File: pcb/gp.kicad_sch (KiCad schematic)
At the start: 31 parts, among them J1 USB-C, SW1 TS-1088R-02526, SW2 TS-1088R-02526, U1 XC6206P332MR, U2 STM32F103CBT6, U3 W25Q32JVSS, Y1 16Mhz

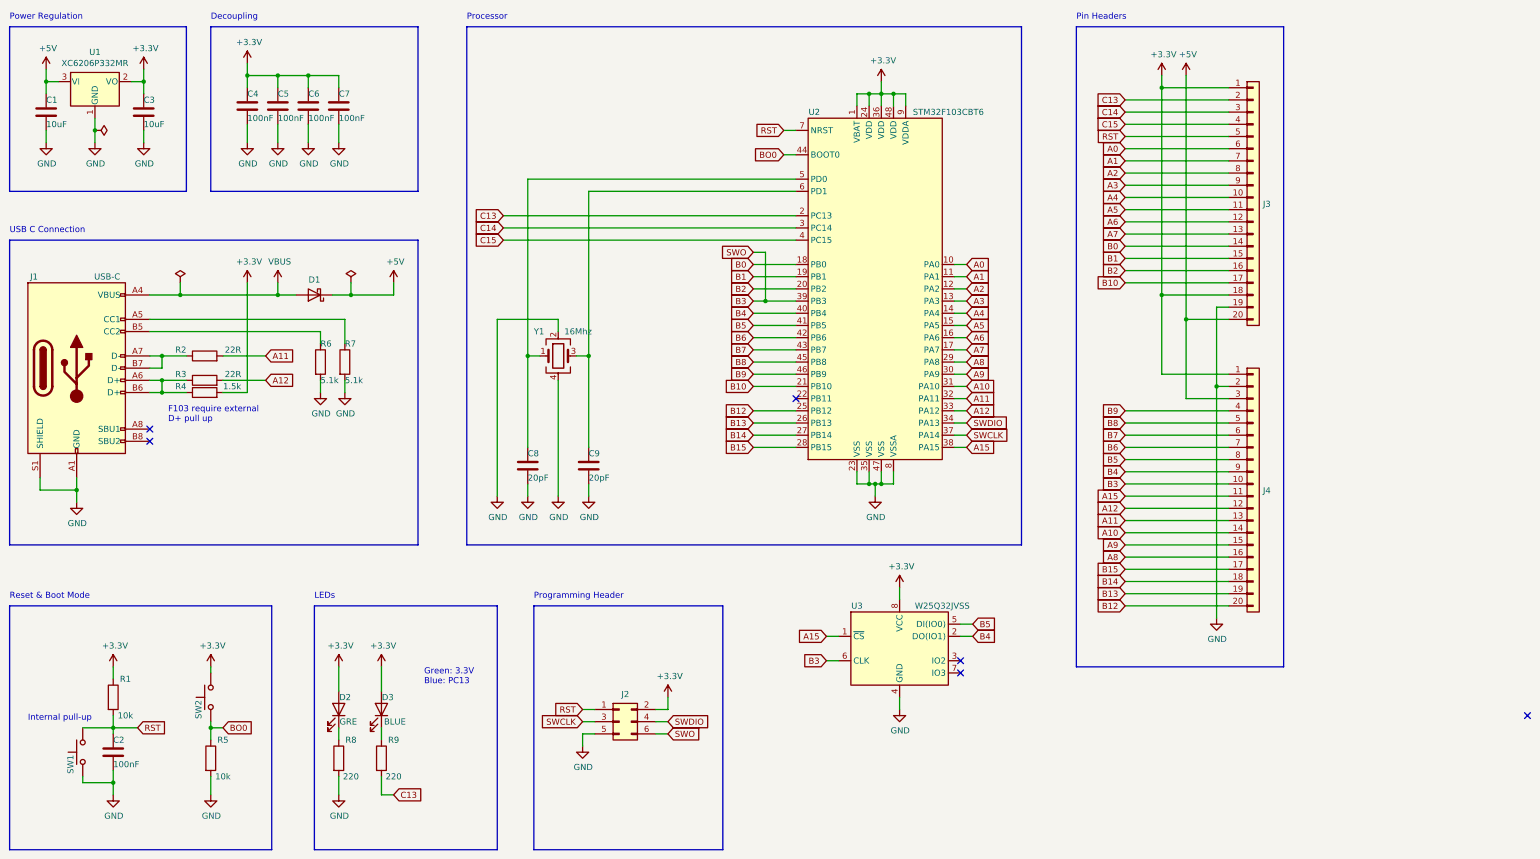
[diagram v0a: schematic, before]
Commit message: Hmmm
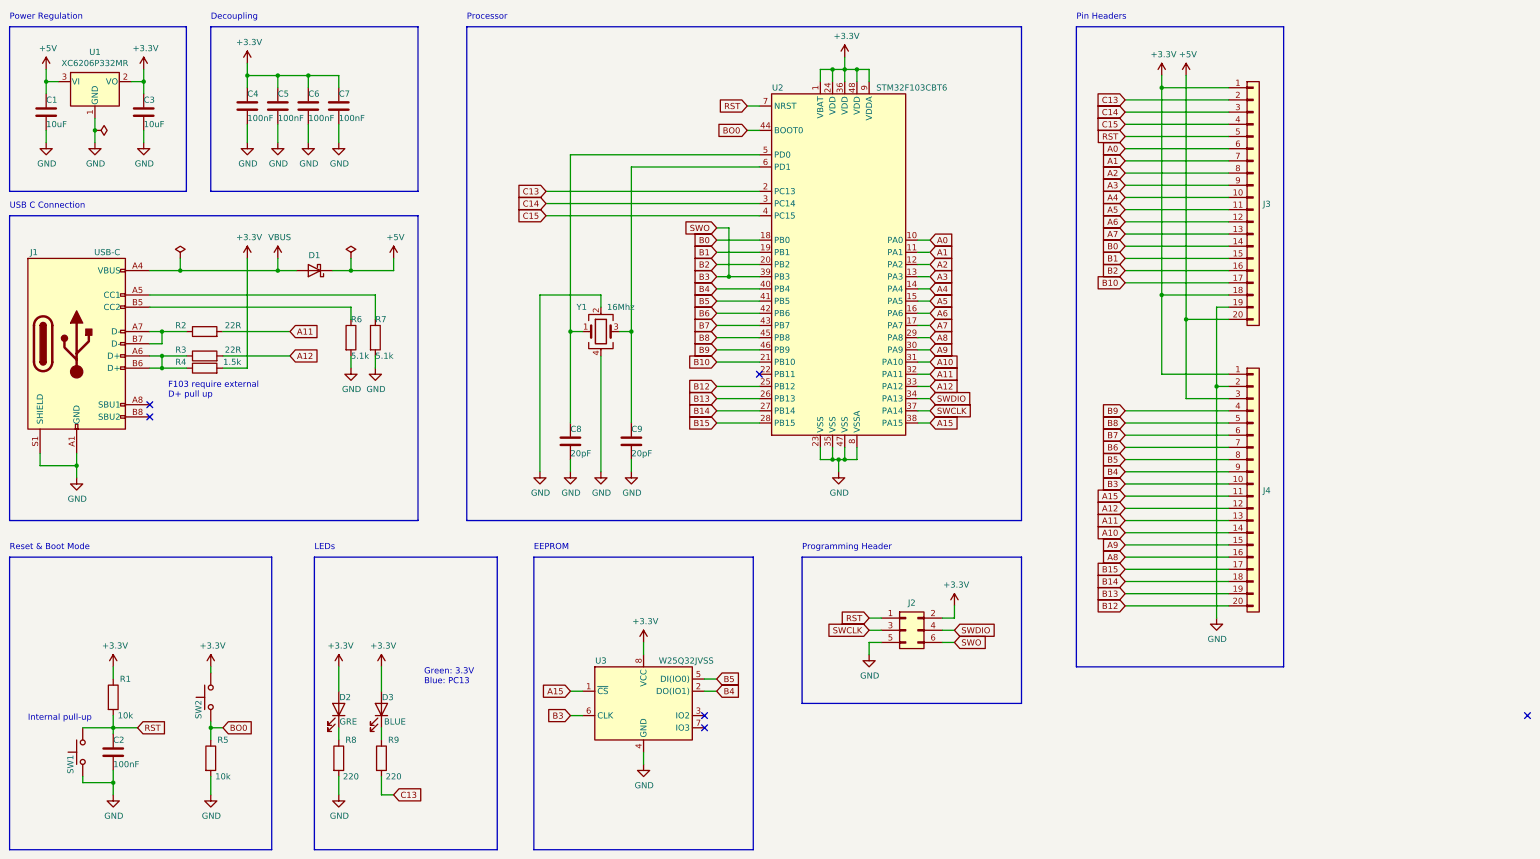
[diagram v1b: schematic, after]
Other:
- note added: "EEPROM"
- moved on the sheet: C8, C9, D1, J1, J2, R2, R3, R4, R6, R7, U2, U3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

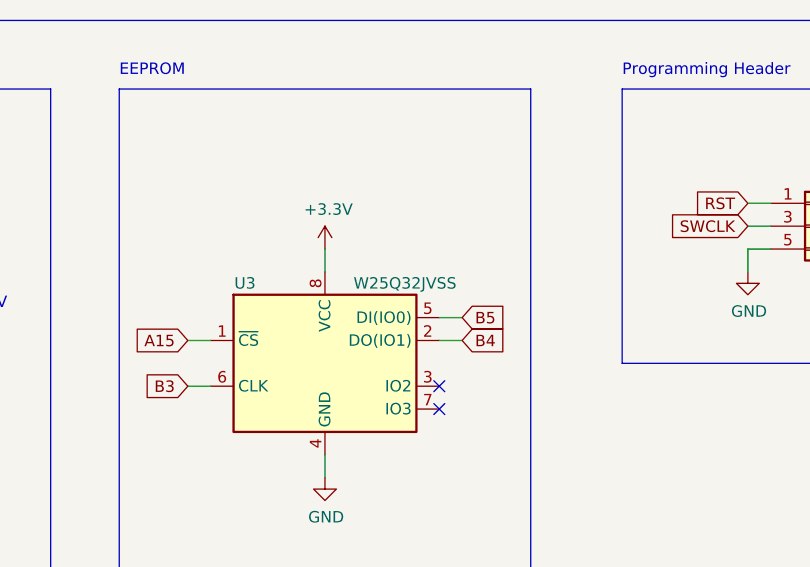
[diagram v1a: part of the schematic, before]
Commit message: Hmmmm
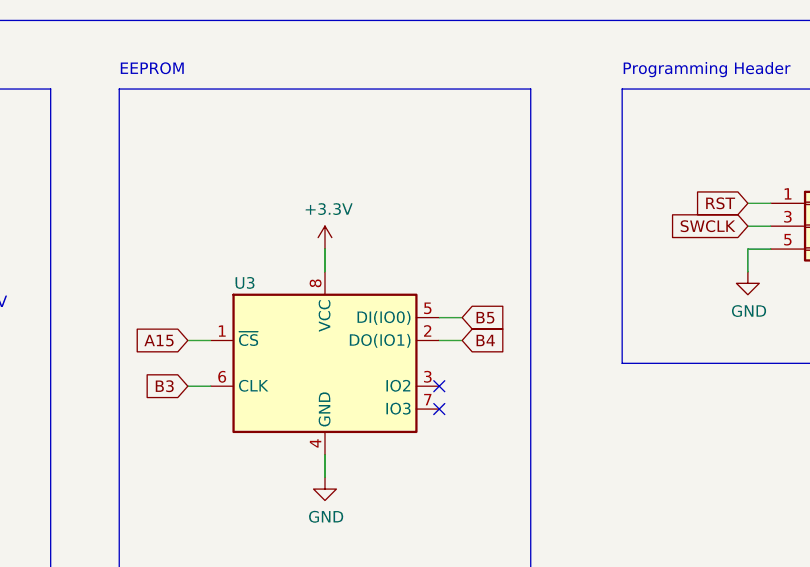
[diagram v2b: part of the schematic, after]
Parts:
- U3: value W25Q32JVSS -> (none); footprint Package_SO:SOIC-8_5.23x5.23mm_P1.27mm -> (none)
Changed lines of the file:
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@@
     (in_bom yes) (on_board yes)
     (property "Reference" "U3" (id 0) (at 137.16 149.86 0))
-    (property "Value" "W25Q32JVSS" (id 1) (at 154.94 149.86 0))
-    (property "Footprint" "Package_SO:SOIC-8_5.23x5.23mm_P1.27mm" (id 2) (at 146.05 158.75 0)
+    (property "Value" "" (id 1) (at 154.94 149.86 0))
+    (property "Footprint" "" (id 2) (at 146.05 158.75 0)
       (effects (font (size 1.27 1.27)) hide)
     )

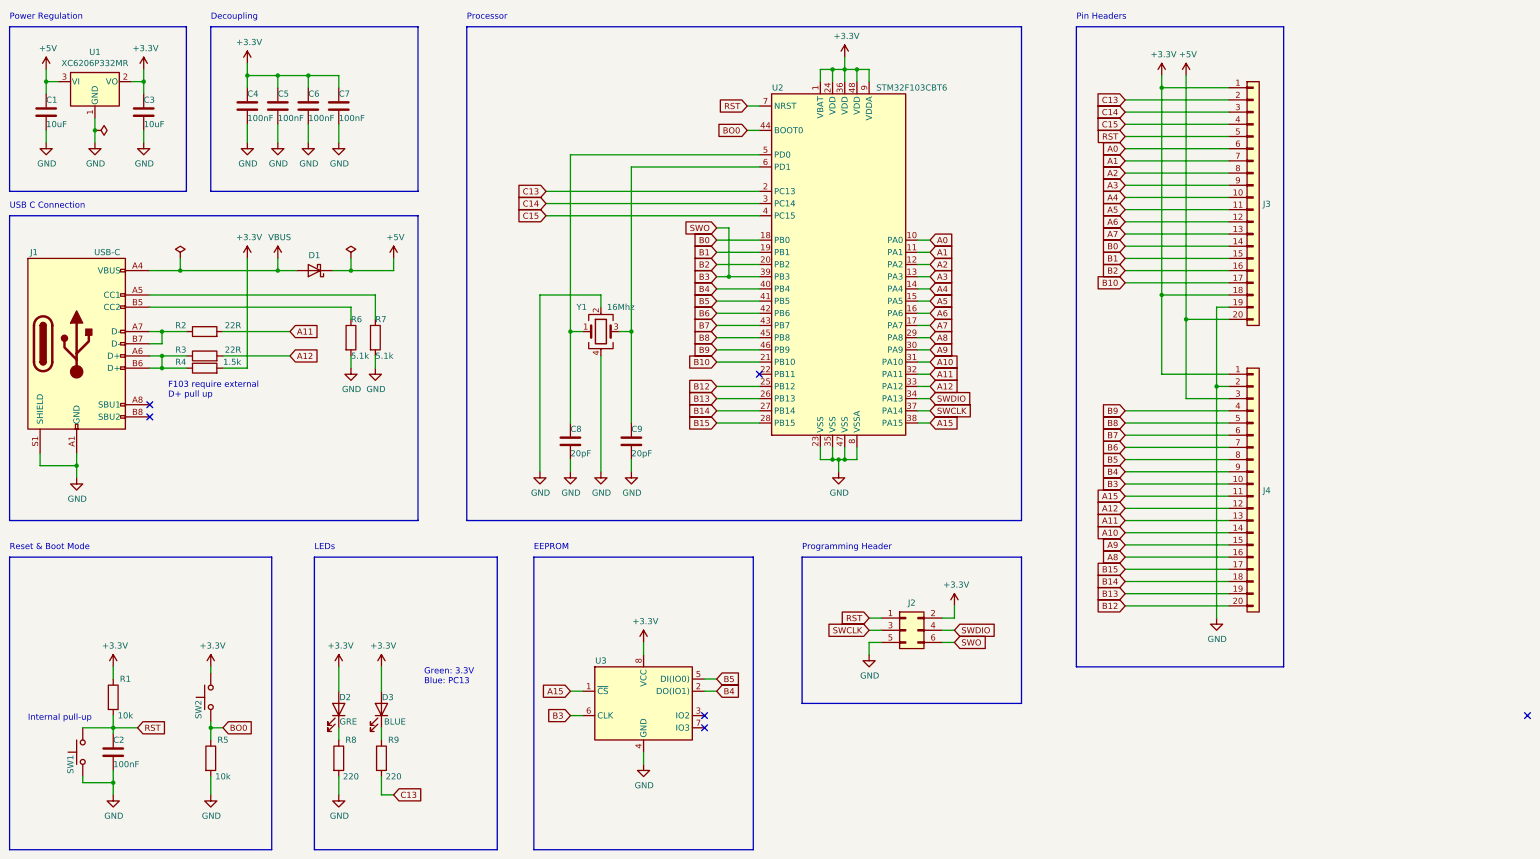
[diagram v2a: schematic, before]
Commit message: Tweaking
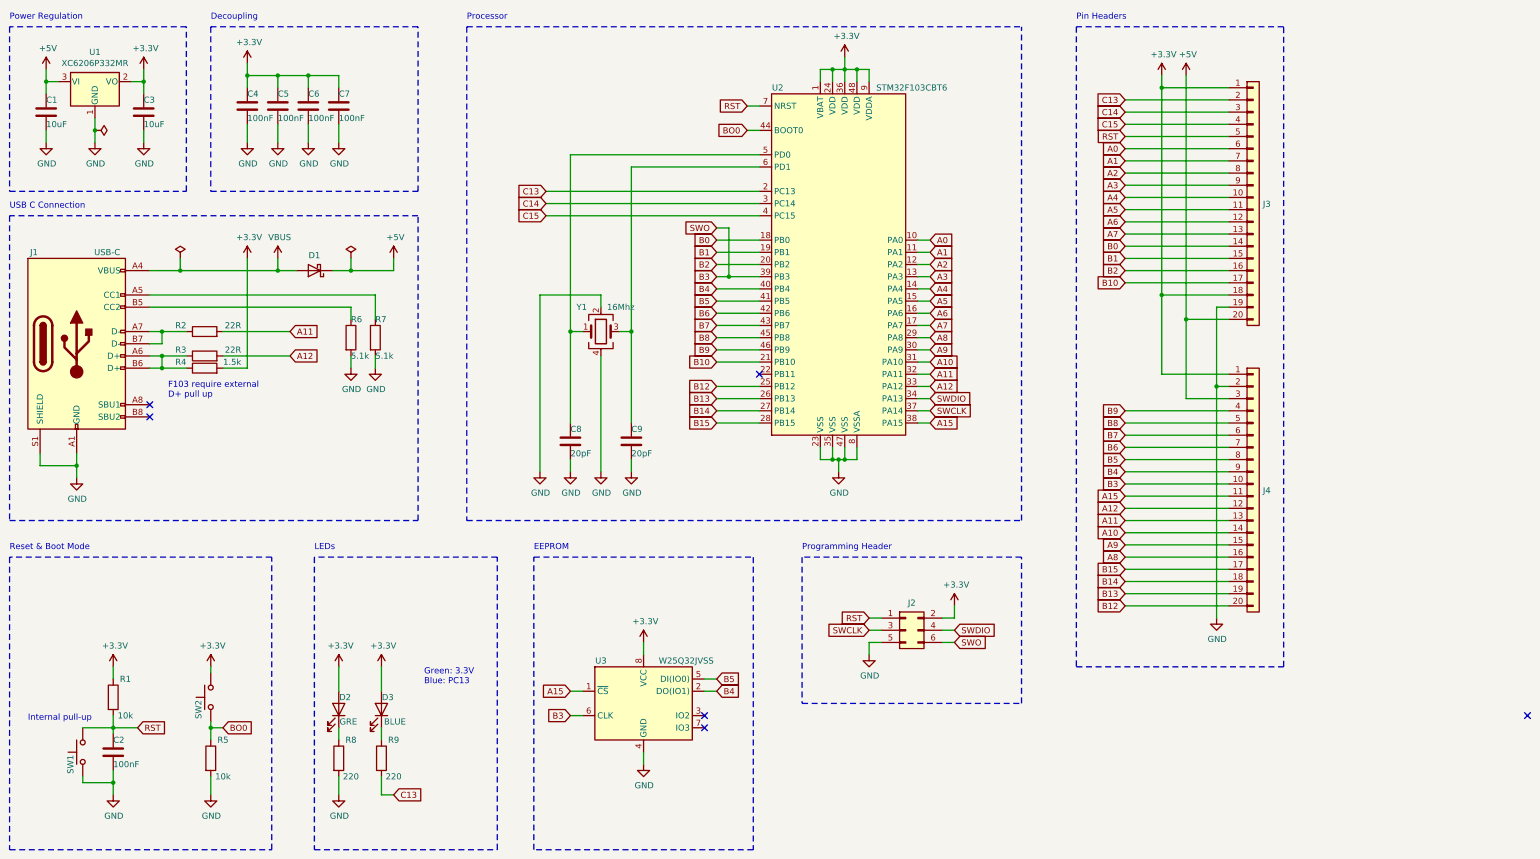
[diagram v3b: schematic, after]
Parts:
- U3: value (none) -> W25Q32JVSS; footprint (none) -> Package_SO:SOIC-8_5.23x5.23mm_P1.27mm

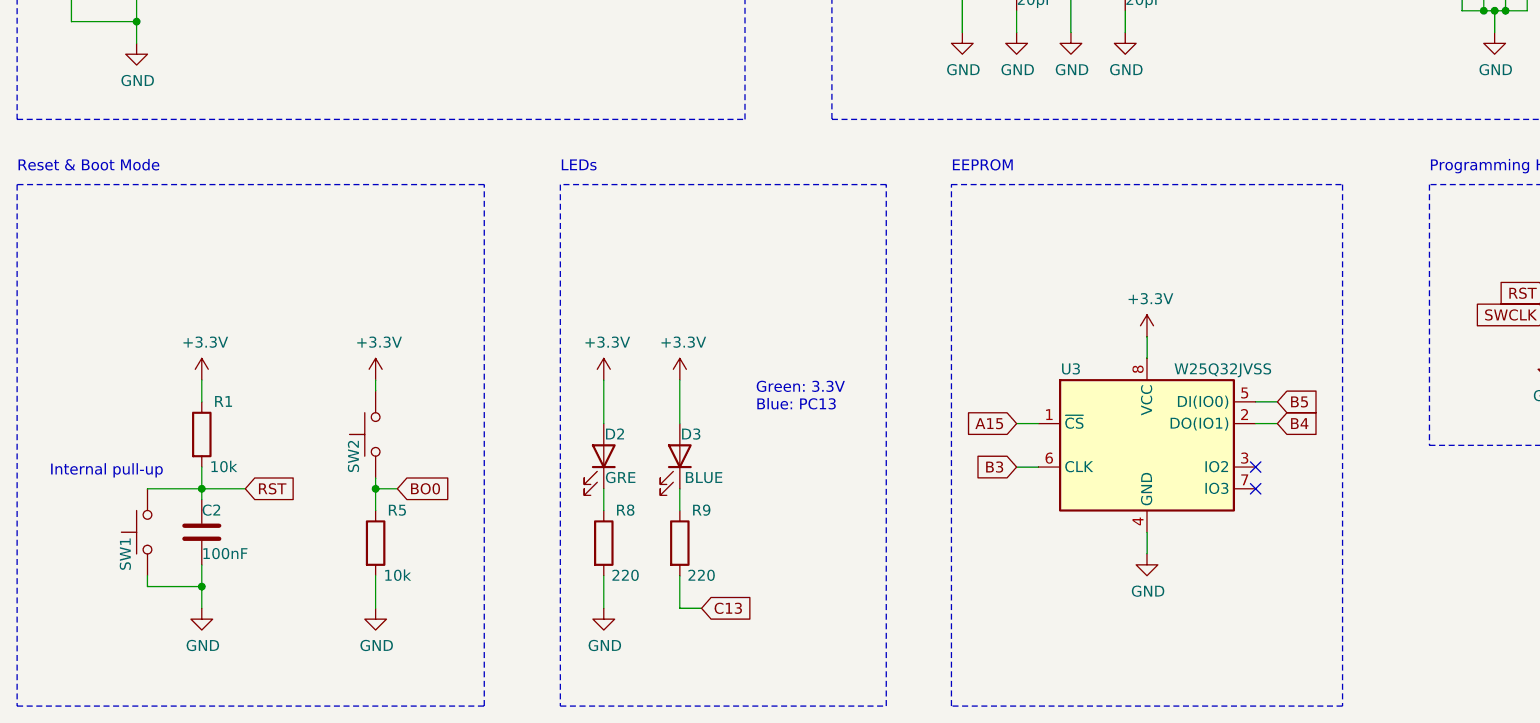
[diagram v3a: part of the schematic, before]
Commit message: Hmmmm
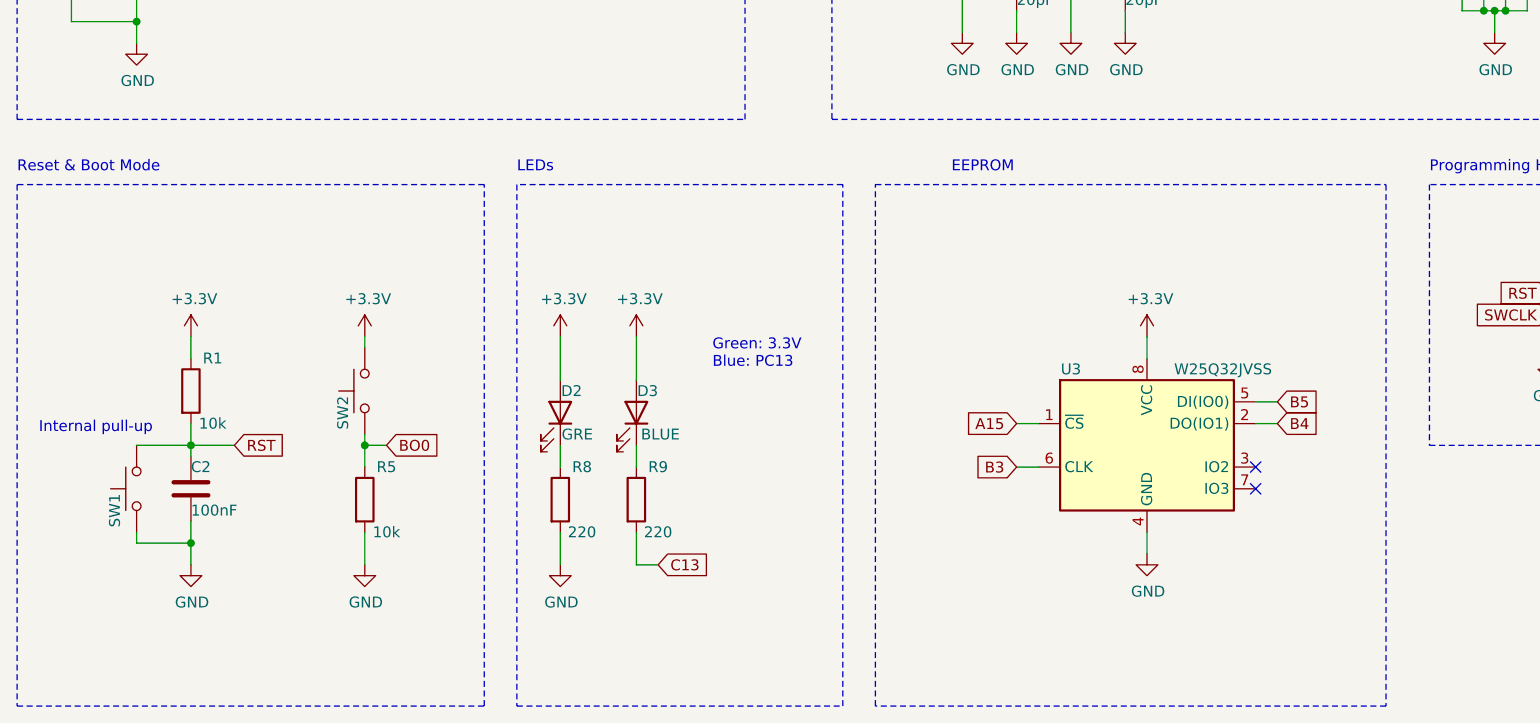
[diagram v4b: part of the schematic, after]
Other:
- moved on the sheet: C2, D2, D3, R1, R5, R8, R9, SW1, SW2
